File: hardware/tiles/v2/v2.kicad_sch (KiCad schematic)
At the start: 29 parts, among them J1 Conn_01x10_Socket, J2 Conn_01x10_Socket, J3 Conn_01x10_Socket, J4 Conn_01x10_Socket, J9 Conn_01x06_Pin, Q1 Q_Photo_NPN_EC, SW1 SW_DIP_x01, U2 DRV5055A2xDBZxQ1, U3 ATmega328-M, Y2 Crystal

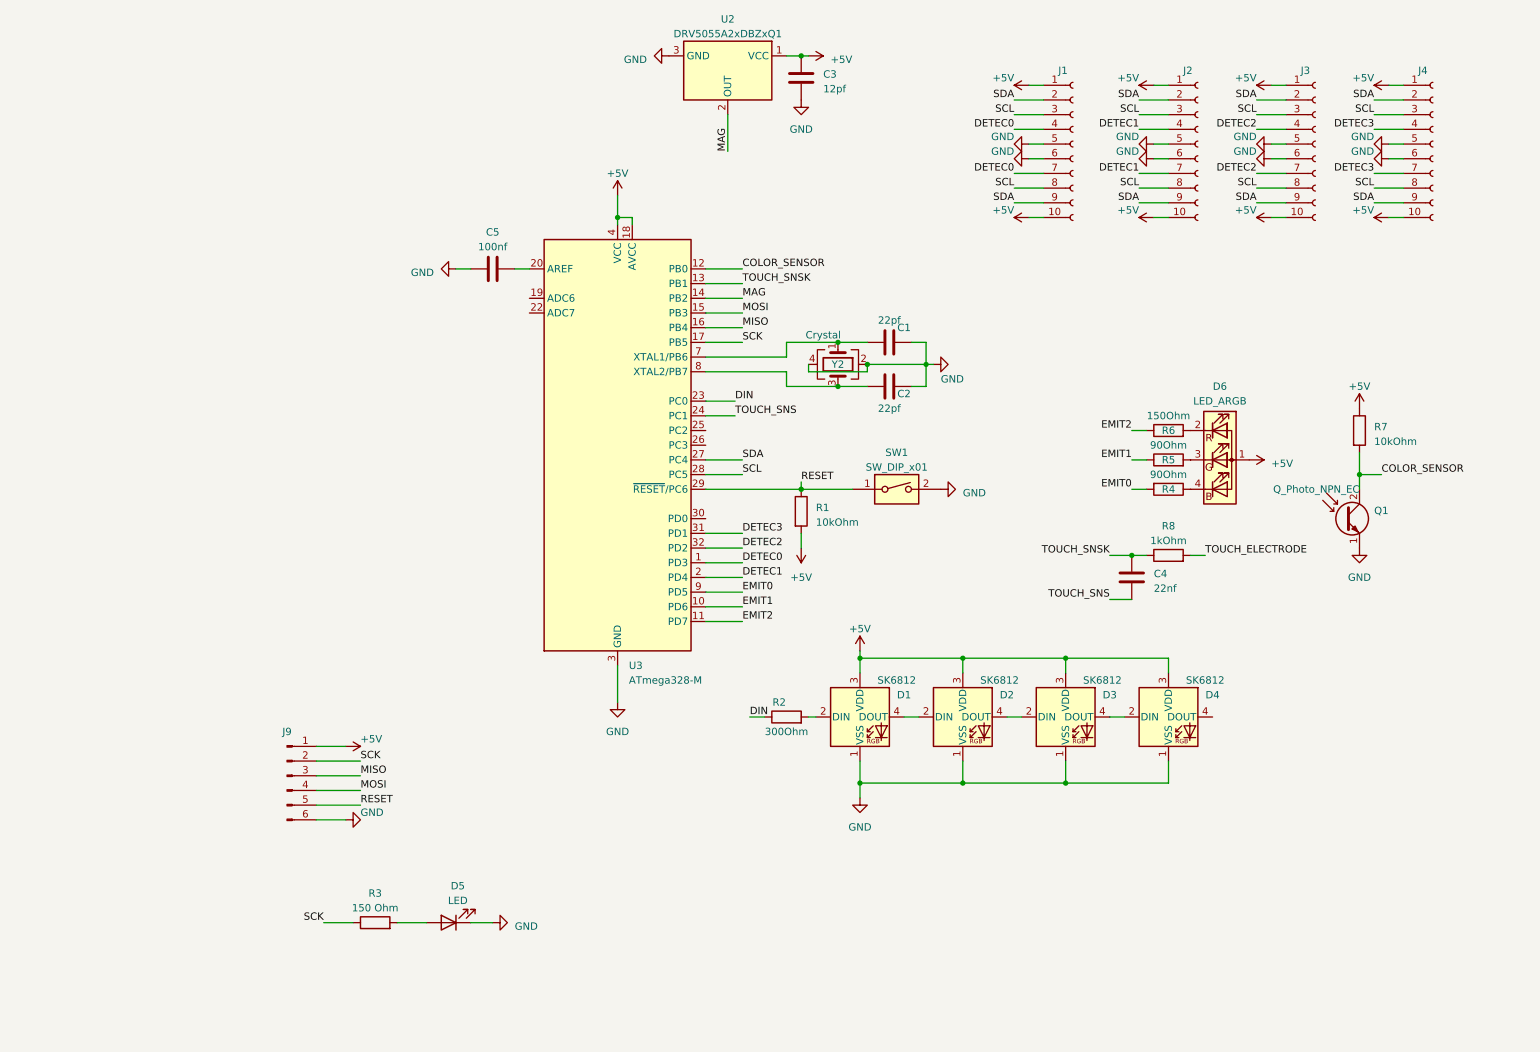
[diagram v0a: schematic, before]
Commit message: Quick save
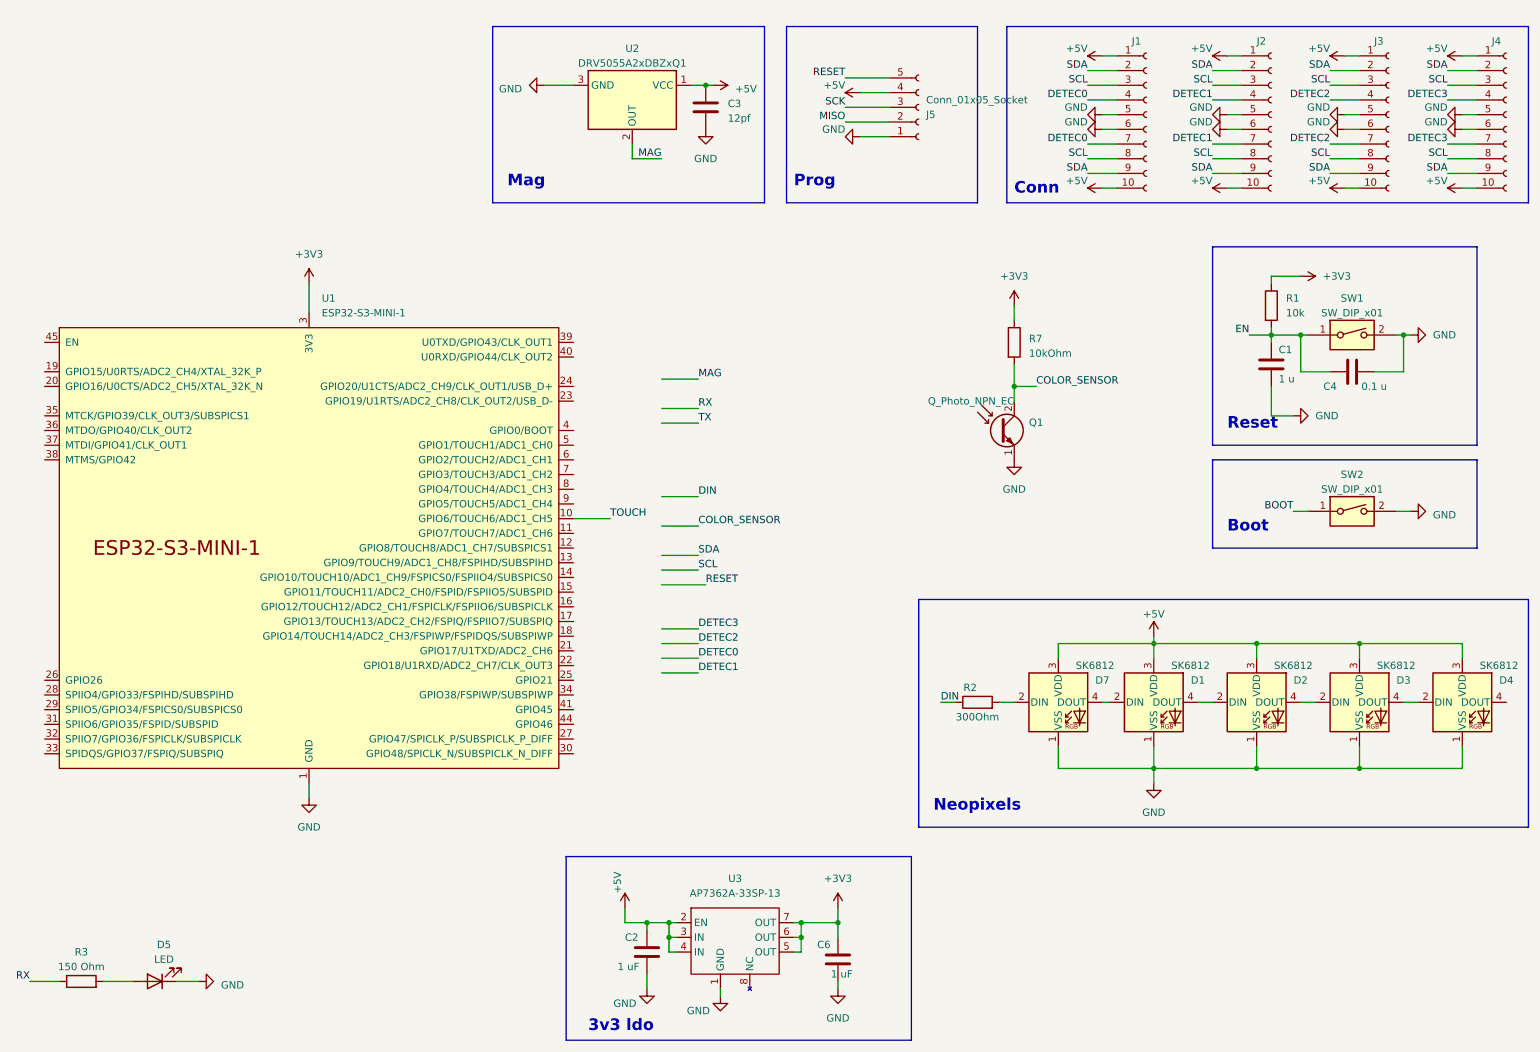
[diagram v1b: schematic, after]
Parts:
- removed C5: 100nf, Capacitor_SMD:C_0603_1608Metric_Pad1.08x0.95mm_HandSolder, symbol Device:C
- removed D6: LED_ARGB, LED_SMD:LED_WS2812B-2020_PLCC4_2.0x2.0mm, symbol Device:LED_ARGB
- removed J9: Conn_01x06_Pin, Connector_PinHeader_2.54mm:PinHeader_1x06_P2.54mm_Vertical, symbol Connector:Conn_01x06_Pin
- removed R4, R5: 90Ohm, Resistor_SMD:R_0603_1608Metric_Pad0.98x0.95mm_HandSolder, symbol Device:R
- removed R6: 150Ohm, Resistor_SMD:R_0603_1608Metric_Pad0.98x0.95mm_HandSolder, symbol Device:R
- removed R8: 1kOhm, Resistor_SMD:R_0603_1608Metric_Pad0.98x0.95mm_HandSolder, symbol Device:R
- removed U3: ATmega328-M, Package_DFN_QFN:QFN-32-1EP_5x5mm_P0.5mm_EP3.1x3.1mm, symbol MCU_Microchip_ATmega:ATmega328-M
- removed Y2: Crystal, Crystal:Crystal_SMD_3225-4Pin_3.2x2.5mm_HandSoldering, symbol Device:Crystal_GND24
- added C6: 1 uF, Capacitor_SMD:C_0603_1608Metric_Pad1.08x0.95mm_HandSolder, symbol Device:C
- added D7: SK6812, LED_SMD:LED_SK6812_PLCC4_5.0x5.0mm_P3.2mm, symbol LED:SK6812
- added J5: Conn_01x05_Socket, Connector_PinSocket_2.54mm:PinSocket_1x05_P2.54mm_Vertical, symbol Connector:Conn_01x05_Socket
- added SW2: SW_DIP_x01, Button_Switch_SMD:SW_Push_1P1T_XKB_TS-1187A, symbol Switch:SW_DIP_x01
- added U1: ESP32-S3-MINI-1, custom:ESP32-S3-MINI-1U, symbol Espressif:ESP32-S3-MINI-1
- added U3: AP7362A-33SP-13, custom:SOIC127P600X163-9N, symbol AP7362A:AP7362A-33SP-13
- C1: value 22pf -> 1 u; footprint Capacitor_SMD:C_0603_1608Metric_Pad1.08x0.95mm_HandSolder -> Capacitor_SMD:C_0603_1608Metric
- C2: value 22pf -> 1 uF
- C4: value 22nf -> 0.1 u; footprint Capacitor_SMD:C_0402_1005Metric_Pad0.74x0.62mm_HandSolder -> Capacitor_SMD:C_0603_1608Metric
- R1: value 10kOhm -> 10k; footprint Resistor_SMD:R_0603_1608Metric_Pad0.98x0.95mm_HandSolder -> Resistor_SMD:R_0603_1608Metric
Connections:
- net TOUCH_SNS is gone; now on net GND: C4.2
- net TOUCH_SNSK is gone; now on net EN: C4.1
- net +5V: now also C2.1, D7.3 (VDD), J5.4 (Pin_4), U3.2 (EN), U3.3 (IN), U3.4 (IN); no longer R1.2, R7.1
- net GND: now also C6.2, D7.1 (VSS), J5.1 (Pin_1), SW2.2, U1.1 (GND), U1.2 (GND), U1.42 (GND), U1.43 (GND), U1.46 (GND), U1.47 (GND), U1.48 (GND), U1.49 (GND), U1.50 (GND), U1.51 (GND), U1.52 (GND), U1.53 (GND), U1.54 (GND), U1.55 (GND), U1.56 (GND), U1.57 (GND), U1.58 (GND), U1.59 (GND), U1.60 (GND), U1.61 (GND), U1.62 (GND), U1.63 (GND), U1.64 (GND), U1.65 (GND), U3.1 (GND)
- net MISO: now also J5.2 (Pin_2)
- net RESET: now also J5.5 (Pin_5); no longer R1.1, SW1.1
- net SCK: now also J5.3 (Pin_3); no longer R3.1
- net EN: now reaches C1.1
- net EN: now also R1.2, SW1.1
- net at R2.2: now also D7.2 (DIN); no longer D1.2 (DIN)
- new net: D1.2 (DIN), D7.4 (DOUT)
- new net +3V3: C6.1, R1.1, R7.1, U1.3 (3V3), U3.5 (OUT), U3.6 (OUT), U3.7 (OUT)
- new net BOOT: SW2.1
- new net RX: R3.1
- new net TOUCH: U1.10 (GPIO6/TOUCH6/ADC1_CH5)
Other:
- note added: "3v3 ldo"
- note added: "Boot"
- note added: "Conn"
- note added: "Mag"
- note added: "Neopixels"
- note added: "Prog"
- note added: "Reset"
- moved on the sheet: C3, D1, D2, D3, D4, D5, J1, J2, J3, J4, Q1, R2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
